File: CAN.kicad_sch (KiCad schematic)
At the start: 4 parts, among them U2 SIT3051

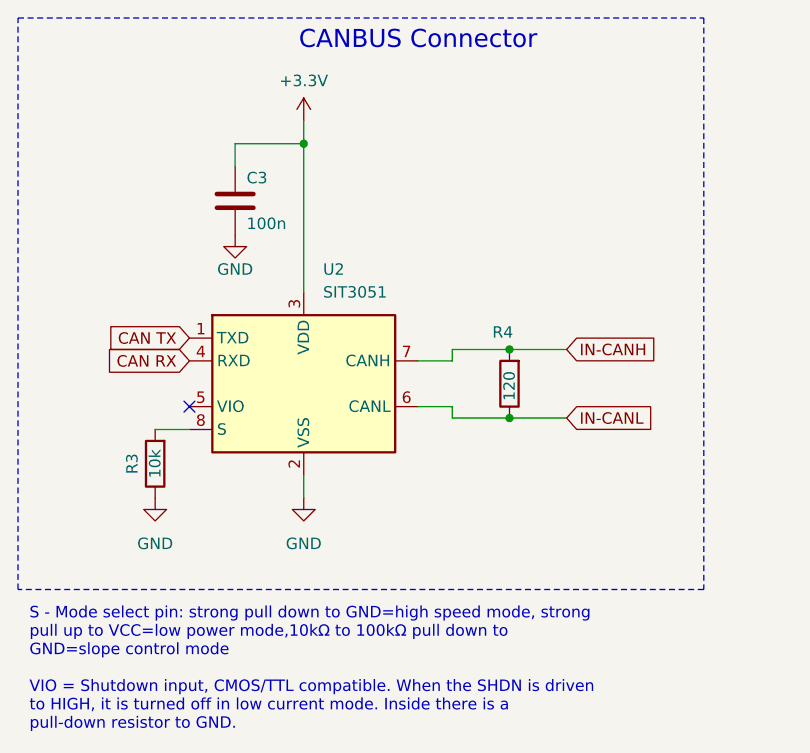
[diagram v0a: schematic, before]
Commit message: initial
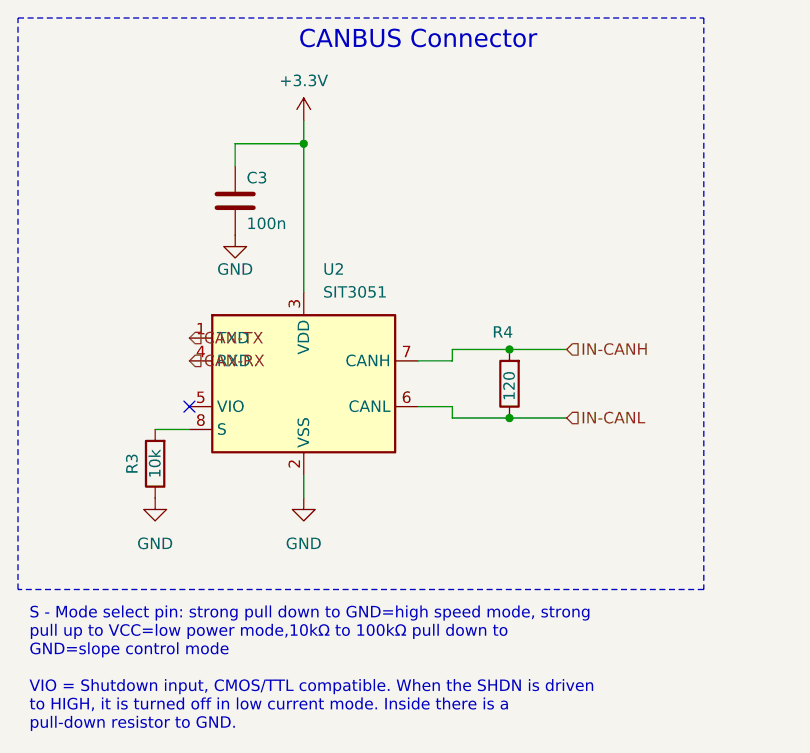
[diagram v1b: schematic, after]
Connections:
- net CAN RX renamed CAN-RX
- net CAN TX renamed CAN-TX
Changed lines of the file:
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@@
 		)
 	)
-	(global_label "CAN RX"
+	(hierarchical_label "CAN-RX"
 		(shape input)
-		(at 116.84 111.76 180)
-		(fields_autoplaced yes)
+		(at 116.84 111.76 0)
 		(effects
 			(font
 				(size 1.27 1.27)
 			)
-			(justify right)
-		)
-		(property "Intersheetrefs" "${INTERSHEET_REFS}"
-			(at 107.4522 111.76 0)
-			(hide yes)
-			(show_name no)
-			(do_not_autoplace no)
-			(effects
-				(font
-					(size 1.27 1.27)
-				)
-				(justify right)
-			)
+			(justify left bottom)
 		)
 	)
-	(global_label "CAN TX"
+	(hierarchical_label "CAN-TX"
 		(shape input)
-		(at 116.84 109.22 180)
-		(fields_autoplaced yes)
+		(at 116.84 109.22 0)
 		(effects
 			(font
 				(size 1.27 1.27)
 			)
-			(justify right)
-		)
-		(property "Intersheetrefs" "${INTERSHEET_REFS}"
-			(at 107.7546 109.22 0)
-			(hide yes)
-			(show_name no)
-			(do_not_autoplace no)
-			(effects
-				(font
-					(size 1.27 1.27)
-				)
-				(justify right)
-			)
+			(justify left bottom)
 		)
 	)
-	(global_label "IN-CANH"
+	(hierarchical_label "IN-CANH"
 		(shape input)
 		(at 158.75 110.49 0)
-		(fields_autoplaced yes)
 		(effects
 			(font
 				(size 1.27 1.27)
 			)
-			(justify left)
-		)
-		(property "Intersheetrefs" "${INTERSHEET_REFS}"
-			(at 169.6083 110.49 0)
-			(hide yes)
-			(show_name no)
-			(do_not_autoplace no)
-			(effects
-				(font
-					(size 1.27 1.27)
-				)
-				(justify left)
-			)
+			(justify left bottom)
 		)
 	)
-	(global_label "IN-CANL"
+	(hierarchical_label "IN-CANL"
 		(shape input)
 		(at 158.75 118.11 0)
-		(fields_autoplaced yes)
 		(effects
 			(font
 				(size 1.27 1.27)
 			)
-			(justify left)
-		)
-		(property "Intersheetrefs" "${INTERSHEET_REFS}"
-			(at 169.3059 118.11 0)
-			(hide yes)
-			(show_name no)
-			(do_not_autoplace no)
-			(effects
-				(font
-					(size 1.27 1.27)
-				)
-				(justify left)
-			)
+			(justify left bottom)
 		)
 	)
